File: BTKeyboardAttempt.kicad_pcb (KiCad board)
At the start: 2 copper layers, 230.5 x 131 mm, 137 parts, among them J1 USB_C_Receptacle, SW1 SW_Push, U2 ATmega32U4-A, Y1 Crystal_GND24_Small

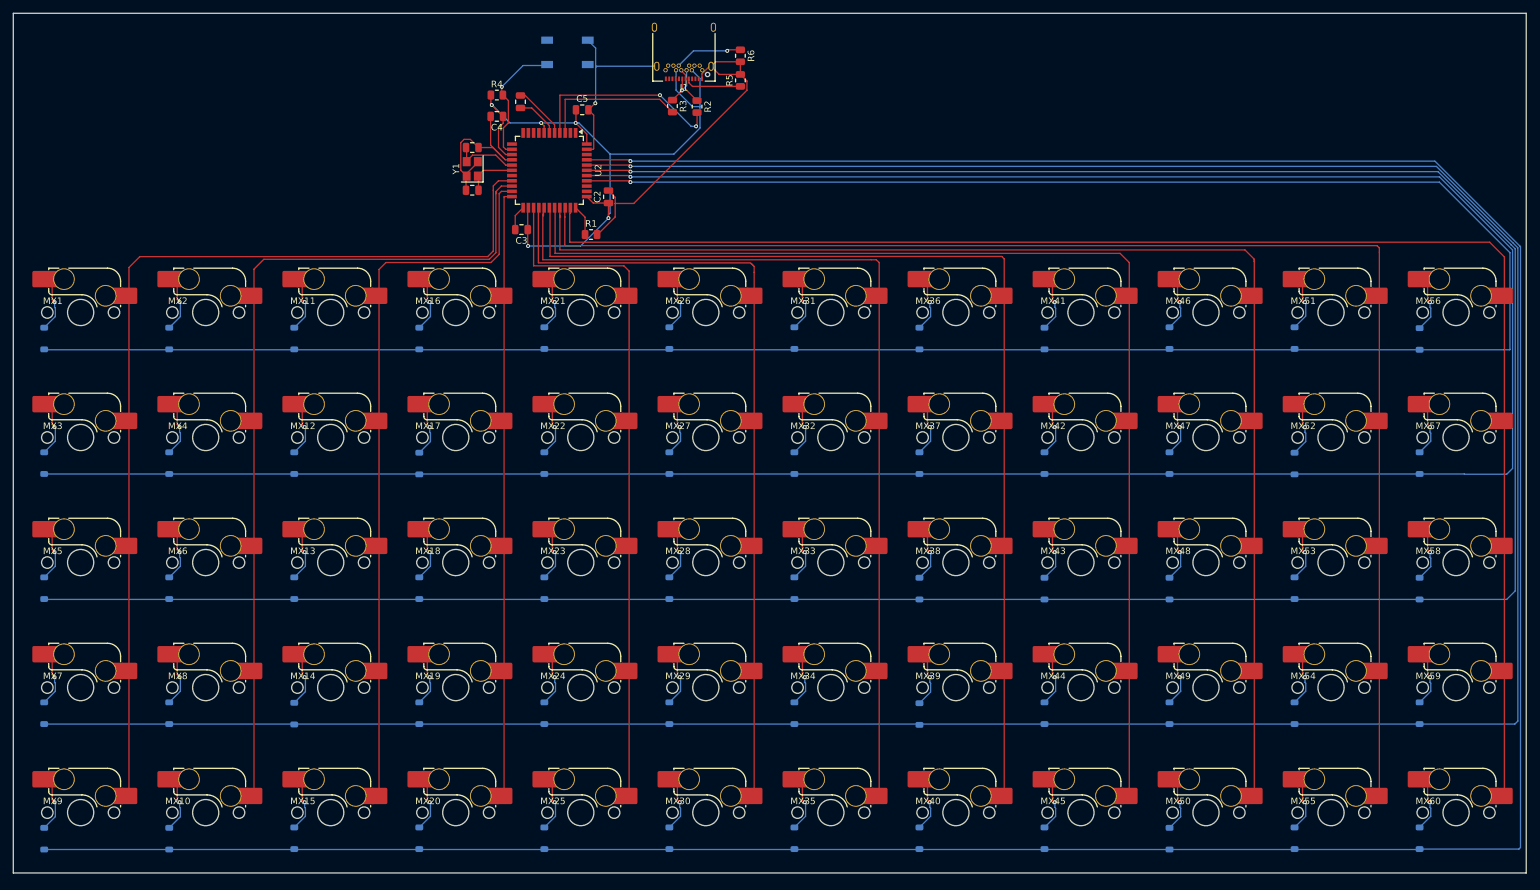
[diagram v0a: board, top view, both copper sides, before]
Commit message: idk what even changed
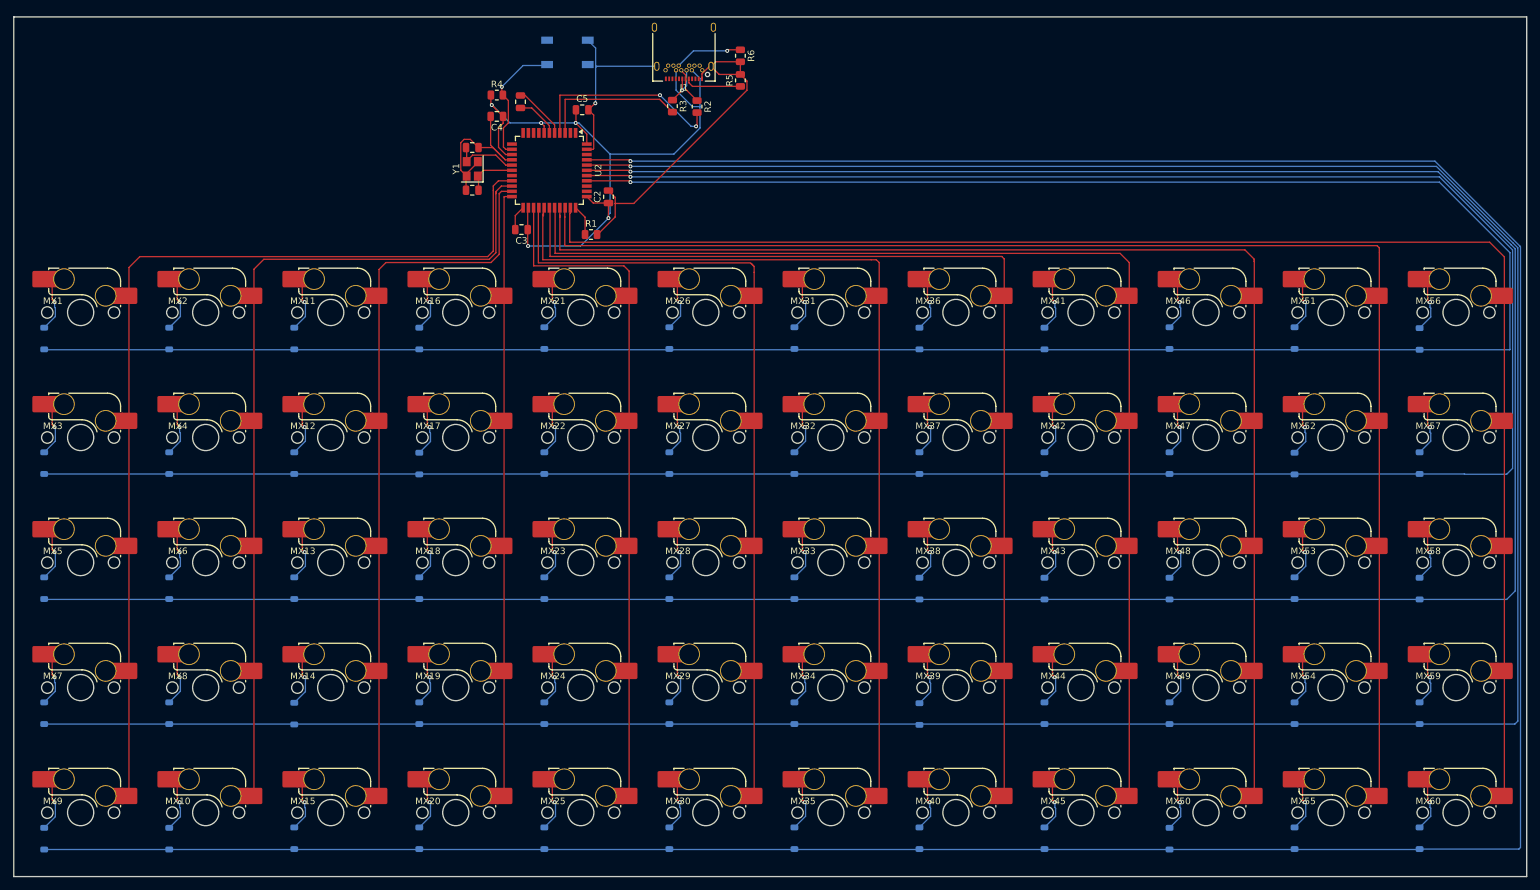
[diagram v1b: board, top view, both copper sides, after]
